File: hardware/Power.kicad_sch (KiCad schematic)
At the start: 3 parts

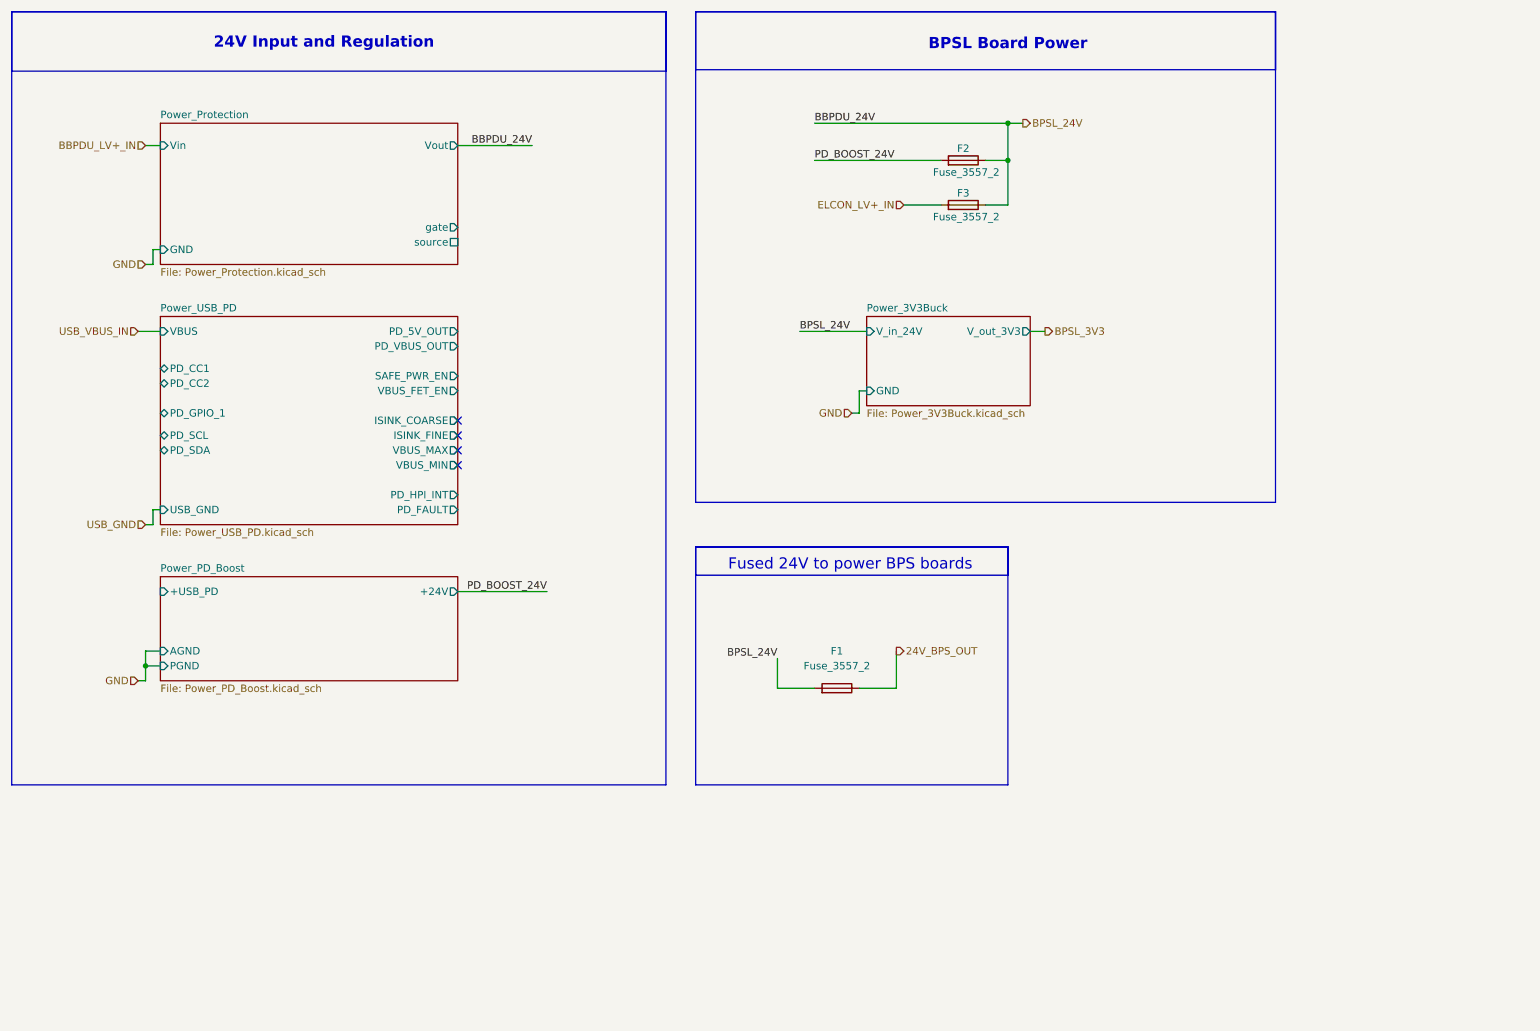
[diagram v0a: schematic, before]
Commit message: power updates
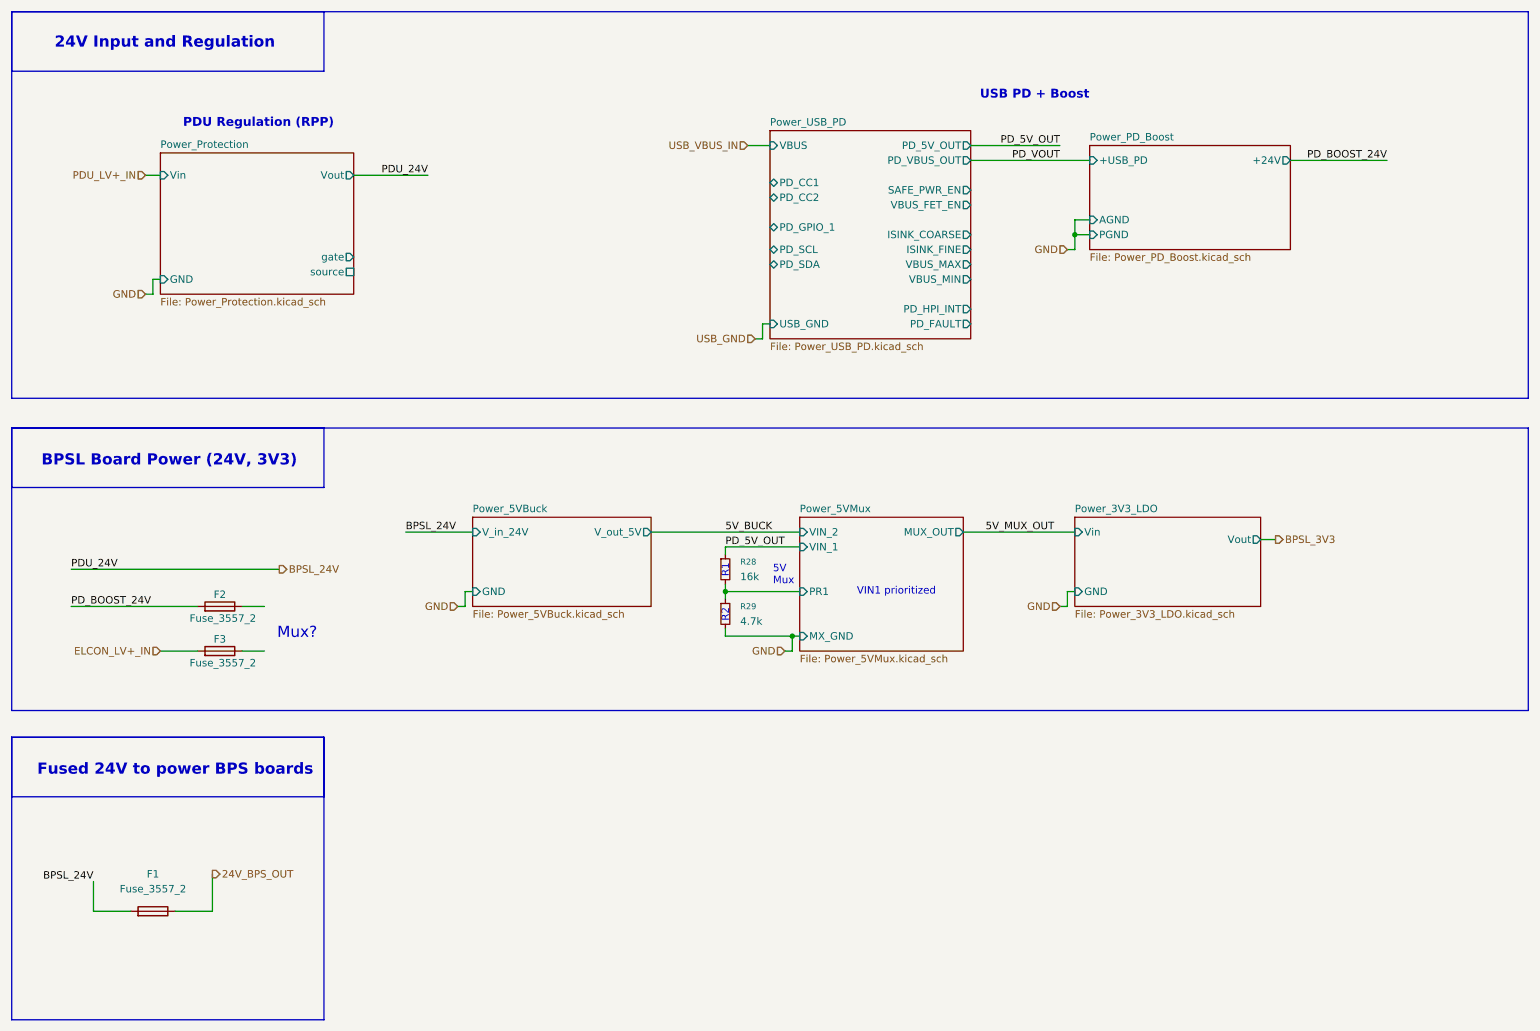
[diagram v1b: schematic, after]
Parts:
- added R28: 16k, symbol Device:R_Small
- added R29: 4.7k, symbol Device:R_Small
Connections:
- net BPSL_24V: no longer F2.2, F3.2
- net GND: now also R29.2
- new net PD_5V_OUT: R28.1
- new net Power_5VMux/PR1: R28.2, R29.1
- no-connect marks 4 -> 0
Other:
- removed sheet Power_3V3Buck
- added sheet Power_3V3_LDO (Power_3V3_LDO.kicad_sch)
- added sheet Power_5VBuck (Power_5VBuck.kicad_sch)
- added sheet Power_5VMux (Power_5VMux.kicad_sch)
- note added: "5V Mux"
- note added: "BPSL Board Power (24V, 3V3)"
- note added: "Mux?"
- note added: "PDU Regulation (RPP)"
- note added: "R1"
- note added: "R2"
- note added: "USB PD + Boost"
- note added: "VIN1 prioritized"
- note removed: "BPSL Board Power"
- moved on the sheet: F1, F2, F3
